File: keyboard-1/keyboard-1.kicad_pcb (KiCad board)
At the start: 2 copper layers, 36 parts, among them J1 Conn_01x12, J2 Conn_01x12, J3 Conn_01x04_Female, SW1 SW_Push, SW10 SW_Push, SW11 SW_Push, SW12 SW_Push, SW13 SW_Push, SW14 SW_Push, SW15 SW_Push, SW16 SW_Push, SW17 SW_Push, SW18 SW_Push, SW19 SW_Push, SW2 SW_Push, SW20 SW_Push, SW21 SW_Push, SW3 SW_Push, SW4 SW_Push, SW5 SW_Push, SW6 SW_Push, SW7 SW_Push, SW8 SW_Push, SW9 SW_Push, U2 TRRS

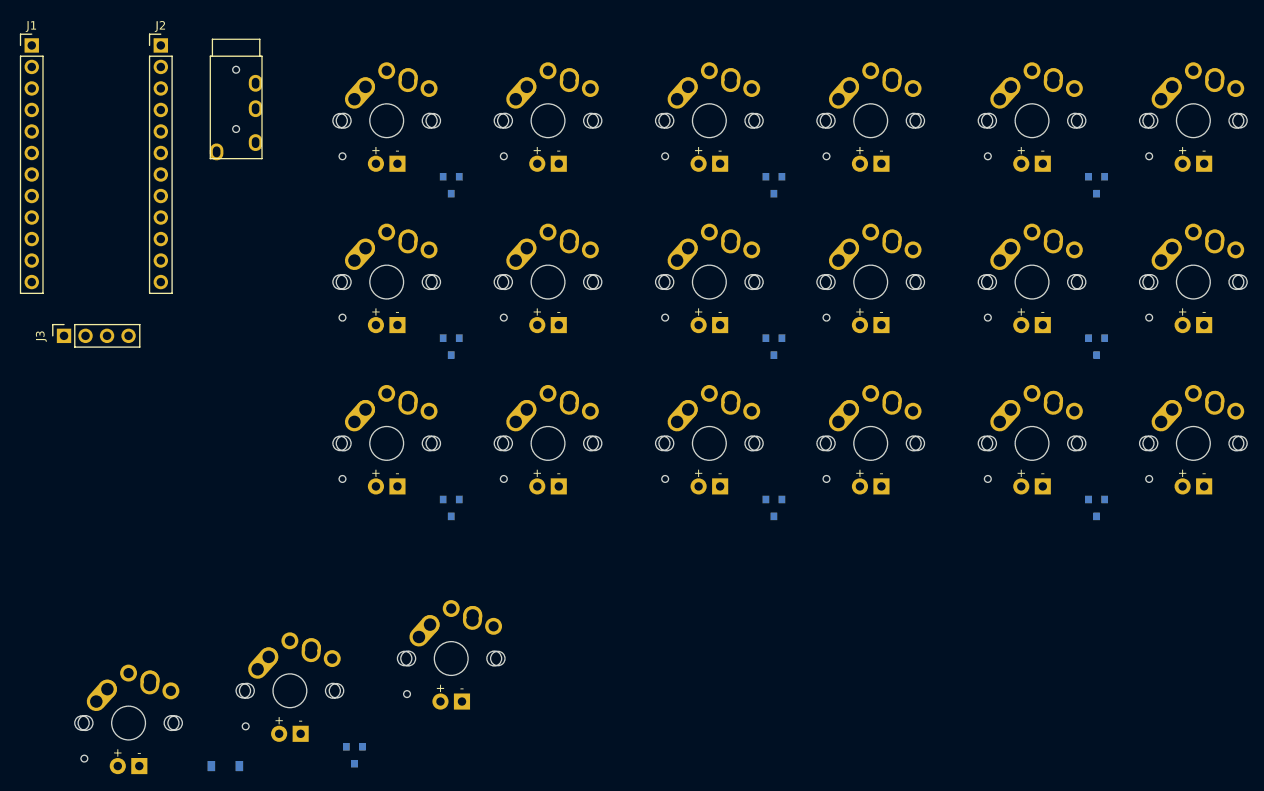
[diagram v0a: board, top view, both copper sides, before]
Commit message: traces to components
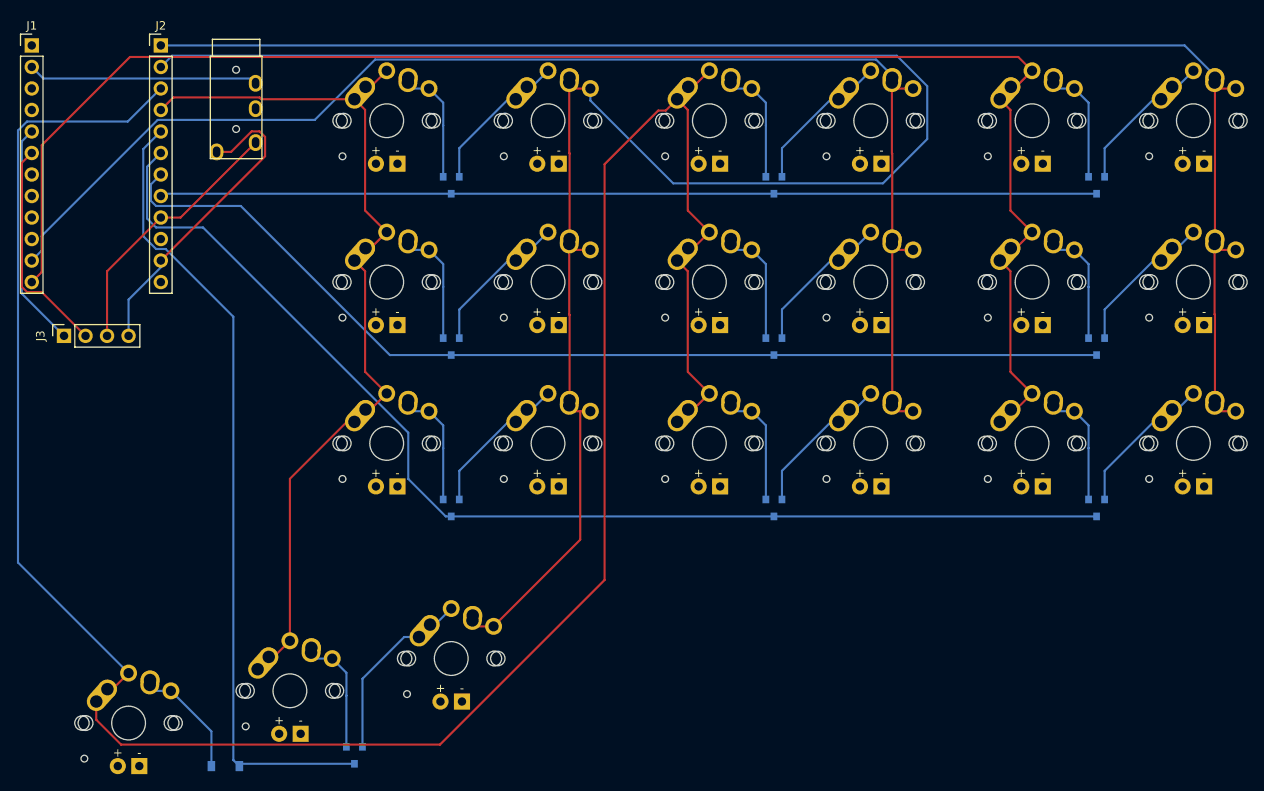
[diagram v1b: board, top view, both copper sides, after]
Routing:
- net /COL2: track 0.00 -> 276.0 mm
- net /COL1: track 0.00 -> 224.6 mm
- net /COL4: track 0.00 -> 188.7 mm
- net /COL5: track 0.00 -> 172.1 mm
- net /COL3: track 0.00 -> 160.6 mm
- net /ROW2: track 0.00 -> 138.3 mm
- net /ROW1: track 0.00 -> 122.8 mm
- net /ROW0: track 0.00 -> 110.6 mm
- net /COL0: track 0.00 -> 108.4 mm
- net /ROW3: track 0.00 -> 94.9 mm
- net GND: track 0.00 -> 37.2 mm
- net VCC: track 0.00 -> 31.5 mm
- net /SERIAL: track 0.00 -> 27.2 mm
- net /SDA: track 0.00 -> 26.7 mm
- net /SCL: track 0.00 -> 26.2 mm
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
